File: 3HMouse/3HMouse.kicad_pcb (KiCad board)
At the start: 2 copper layers, 204.8 x 104.8 mm, 85 parts, among them J1 USB_C_Receptacle_USB2.0, SW1 CherryMX, SW10 CherryMX, SW11 CherryMX, SW12 CherryMX, SW13 CherryMX, SW14 CherryMX, SW15 CherryMX, SW16 CherryMX, SW17 CherryMX, SW18 CherryMX, SW19 CherryMX, SW2 CherryMX, SW20 CherryMX, SW21 CherryMX, SW22 CherryMX, SW23 CherryMX, SW24 CherryMX, SW25 CherryMX, SW26 CherryMX, SW27 CherryMX, SW28 CherryMX, SW29 CherryMX, SW3 CherryMX, SW30 RotaryEncoder, SW31 RotaryEncoder, SW4 CherryMX, SW5 CherryMX, SW6 CherryMX, SW7 CherryMX, SW8 CherryMX, SW9 CherryMX, U1 ATmega32U4-M, U2 USBLC6-2SC6, Y1 16 MHz

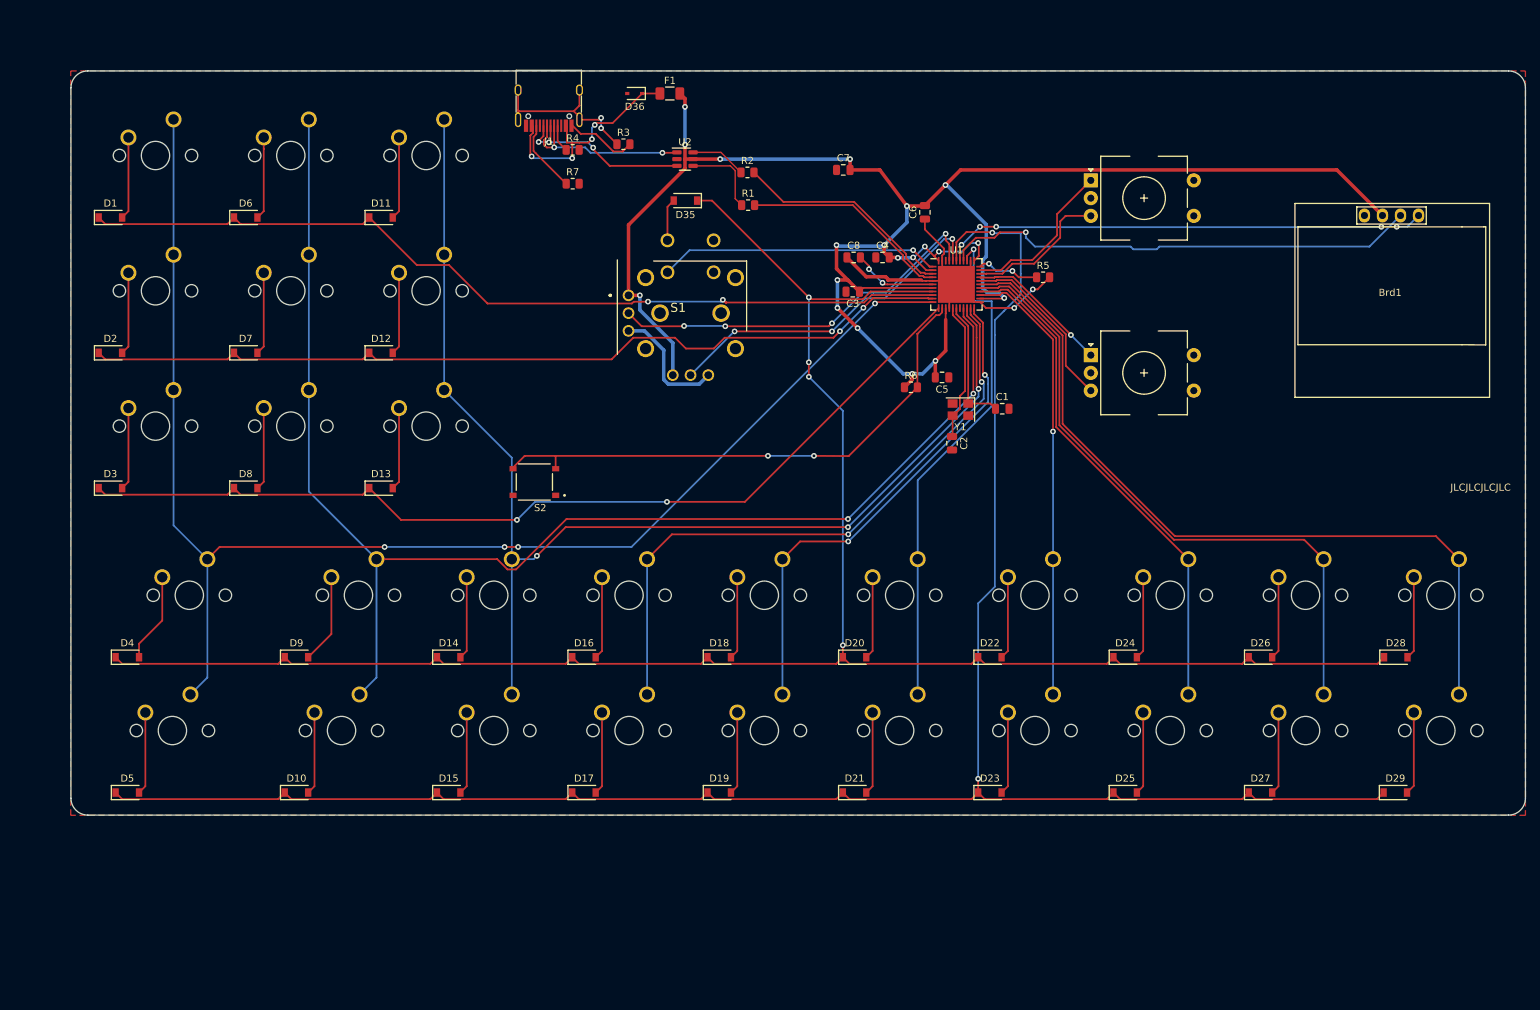
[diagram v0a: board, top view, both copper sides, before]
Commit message: Placements done for v2
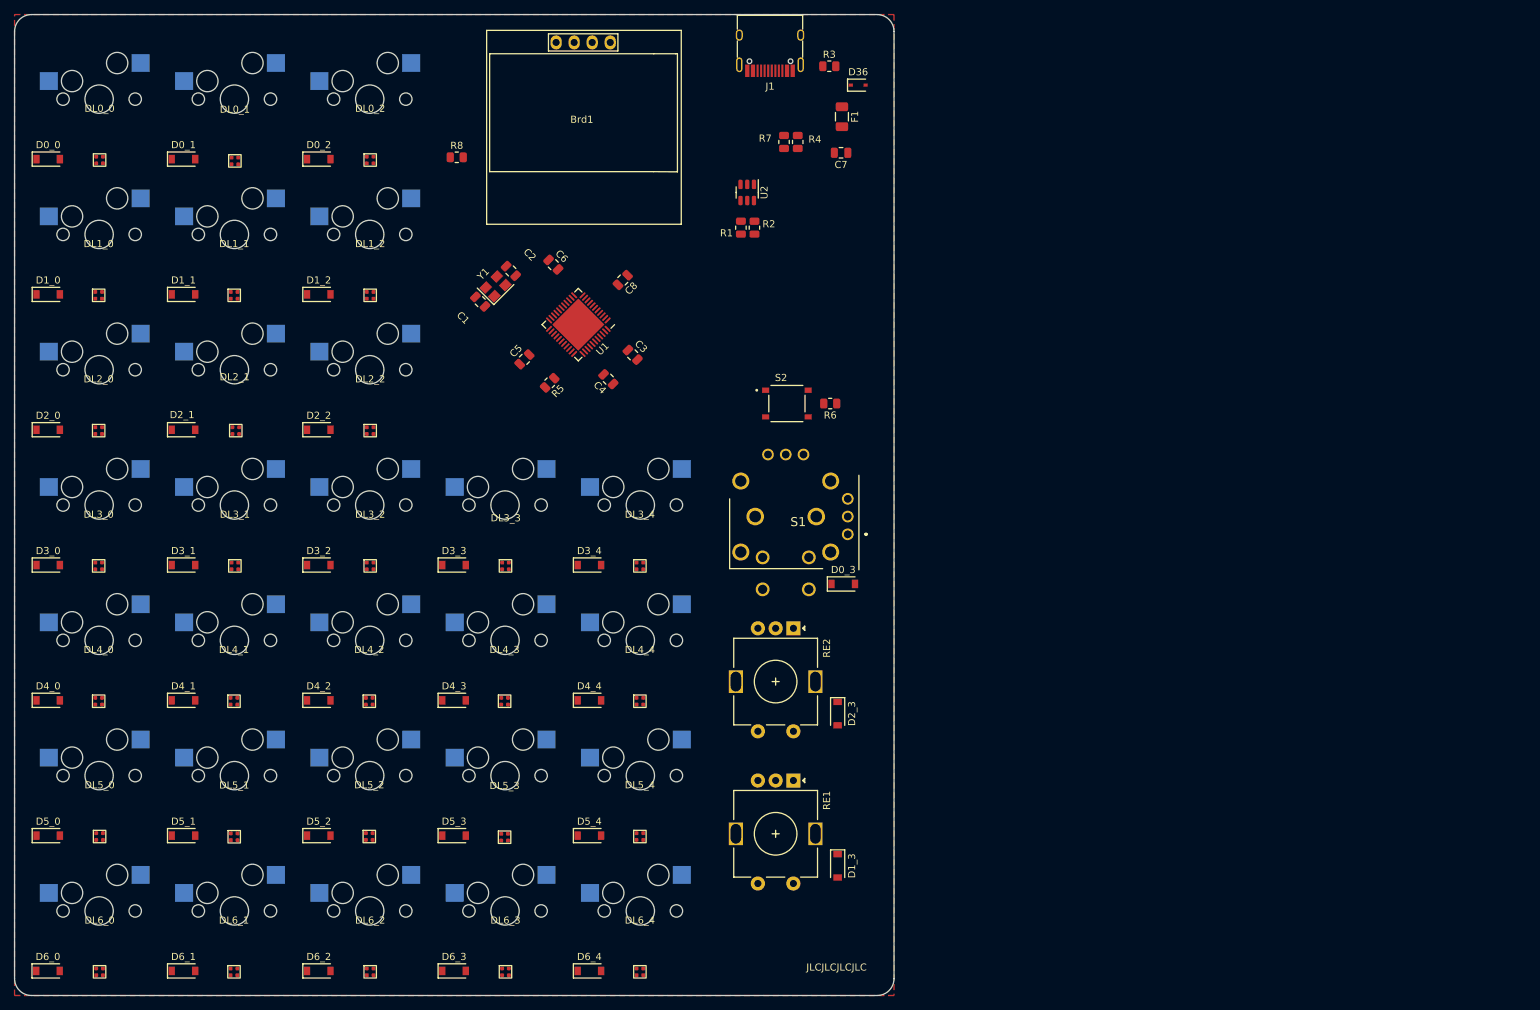
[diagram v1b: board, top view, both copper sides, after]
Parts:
- removed D1, D10, D11, D12, D13, D14, D15, D16, D17, D18, D19, D2, D20, D21, D22, D23, D24, D25, D26, D27, D28, D29, D3, D35, D4, D5, D6, D7, D8, D9: D_Small, Diode_SMD:D_SOD-123
- removed SW1, SW11, SW12, SW13, SW14, SW15, SW16, SW17, SW18, SW19, SW2, SW20, SW21, SW22, SW23, SW24, SW25, SW26, SW27, SW28, SW29, SW3, SW6, SW7, SW8, SW9: CherryMX, MX_Only:MXOnly-1U-NoLED
- removed SW10, SW5: CherryMX, MX_Only:MXOnly-1.25U-NoLED
- removed SW30, SW31: RotaryEncoder, Keebio-Parts:RotaryEncoder_EC11
- removed SW4: CherryMX, MX_Only:MXOnly-1.5U-NoLED
- added D0_0: D_Small, Diode_SMD:D_SOD-123, F.Cu at (26.2, 41.8)
- added D0_1: D_Small, Diode_SMD:D_SOD-123, F.Cu at (45.2, 41.8)
- added D0_2: D_Small, Diode_SMD:D_SOD-123, F.Cu at (64.3, 41.8)
- added D0_3: D_Small, Diode_SMD:D_SOD-123, F.Cu at (138.1, 101.6)
- added D1_0: D_Small, Diode_SMD:D_SOD-123, F.Cu at (26.2, 60.8)
- added D1_1: D_Small, Diode_SMD:D_SOD-123, F.Cu at (45.2, 60.8)
- added D1_2: D_Small, Diode_SMD:D_SOD-123, F.Cu at (64.3, 60.8)
- added D1_3: D_Small, Diode_SMD:D_SOD-123, F.Cu at (137.3, 141.3)
- added D2_0: D_Small, Diode_SMD:D_SOD-123, F.Cu at (26.2, 79.9)
- added D2_1: D_Small, Diode_SMD:D_SOD-123, F.Cu at (45.2, 79.9)
- added D2_2: D_Small, Diode_SMD:D_SOD-123, F.Cu at (64.3, 79.9)
- added D2_3: D_Small, Diode_SMD:D_SOD-123, F.Cu at (137.3, 119.9)
- added D3_0: D_Small, Diode_SMD:D_SOD-123, F.Cu at (26.2, 98.9)
- added D3_1: D_Small, Diode_SMD:D_SOD-123, F.Cu at (45.2, 98.9)
- added D3_2: D_Small, Diode_SMD:D_SOD-123, F.Cu at (64.3, 98.9)
- added D3_3: D_Small, Diode_SMD:D_SOD-123, F.Cu at (83.3, 98.9)
- added D3_4: D_Small, Diode_SMD:D_SOD-123, F.Cu at (102.4, 98.9)
- added D4_0: D_Small, Diode_SMD:D_SOD-123, F.Cu at (26.2, 118.0)
- added D4_1: D_Small, Diode_SMD:D_SOD-123, F.Cu at (45.2, 118.0)
- added D4_2: D_Small, Diode_SMD:D_SOD-123, F.Cu at (64.3, 118.0)
- added D4_3: D_Small, Diode_SMD:D_SOD-123, F.Cu at (83.3, 118.0)
- added D4_4: D_Small, Diode_SMD:D_SOD-123, F.Cu at (102.4, 118.0)
- added D5_0: D_Small, Diode_SMD:D_SOD-123, F.Cu at (26.2, 137.0)
- added D5_1: D_Small, Diode_SMD:D_SOD-123, F.Cu at (45.2, 137.0)
- added D5_2: D_Small, Diode_SMD:D_SOD-123, F.Cu at (64.3, 137.0)
- added D5_3: D_Small, Diode_SMD:D_SOD-123, F.Cu at (83.3, 137.0)
- added D5_4: D_Small, Diode_SMD:D_SOD-123, F.Cu at (102.4, 137.0)
- added D6_0: D_Small, Diode_SMD:D_SOD-123, F.Cu at (26.1, 156.1)
- added D6_1: D_Small, Diode_SMD:D_SOD-123, F.Cu at (45.2, 156.1)
- added D6_2: D_Small, Diode_SMD:D_SOD-123, F.Cu at (64.3, 156.1)
- added D6_3: D_Small, Diode_SMD:D_SOD-123, F.Cu at (83.3, 156.1)
- added D6_4: D_Small, Diode_SMD:D_SOD-123, F.Cu at (102.4, 156.1)
- added DL0_0: SK6805-EC15, HLibrary:SK6805-EC15, F.Cu at (33.4, 41.9)
- added DL0_1: SK6805-EC15, HLibrary:SK6805-EC15, F.Cu at (52.5, 42.0)
- added DL0_2: SK6805-EC15, HLibrary:SK6805-EC15, F.Cu at (71.5, 41.9)
- added DL1_0: SK6805-EC15, HLibrary:SK6805-EC15, F.Cu at (33.3, 61.0)
- added DL1_1: SK6805-EC15, HLibrary:SK6805-EC15, F.Cu at (52.4, 61.0)
- added DL1_2: SK6805-EC15, HLibrary:SK6805-EC15, F.Cu at (71.5, 61.0)
- added DL2_0: SK6805-EC15, HLibrary:SK6805-EC15, F.Cu at (33.3, 80.0)
- added DL2_1: SK6805-EC15, HLibrary:SK6805-EC15, F.Cu at (52.6, 80.0)
- added DL2_2: SK6805-EC15, HLibrary:SK6805-EC15, F.Cu at (71.5, 80.0)
- added DL3_0: SK6805-EC15, HLibrary:SK6805-EC15, F.Cu at (33.3, 99.1)
- added DL3_1: SK6805-EC15, HLibrary:SK6805-EC15, F.Cu at (52.5, 99.1)
- added DL3_2: SK6805-EC15, HLibrary:SK6805-EC15, F.Cu at (71.5, 99.1)
- added DL3_3: SK6805-EC15, HLibrary:SK6805-EC15, F.Cu at (90.6, 99.1)
- added DL3_4: SK6805-EC15, HLibrary:SK6805-EC15, F.Cu at (109.5, 99.1)
- added DL4_0: SK6805-EC15, HLibrary:SK6805-EC15, F.Cu at (33.3, 118.1)
- added DL4_1: SK6805-EC15, HLibrary:SK6805-EC15, F.Cu at (52.3, 118.1)
- added DL4_2: SK6805-EC15, HLibrary:SK6805-EC15, F.Cu at (71.4, 118.1)
- added DL4_3: SK6805-EC15, HLibrary:SK6805-EC15, F.Cu at (90.4, 118.1)
- added DL4_4: SK6805-EC15, HLibrary:SK6805-EC15, F.Cu at (109.5, 118.1)
- added DL5_0: SK6805-EC15, HLibrary:SK6805-EC15, F.Cu at (33.4, 137.2)
- added DL5_1: SK6805-EC15, HLibrary:SK6805-EC15, F.Cu at (52.4, 137.2)
- added DL5_2: SK6805-EC15, HLibrary:SK6805-EC15, F.Cu at (71.4, 137.2)
- added DL5_3: SK6805-EC15, HLibrary:SK6805-EC15, F.Cu at (90.4, 137.3)
- added DL5_4: SK6805-EC15, HLibrary:SK6805-EC15, F.Cu at (109.5, 137.2)
- added DL6_0: SK6805-EC15, HLibrary:SK6805-EC15, F.Cu at (33.4, 156.2)
- added DL6_1: SK6805-EC15, HLibrary:SK6805-EC15, F.Cu at (52.3, 156.2)
- added DL6_2: SK6805-EC15, HLibrary:SK6805-EC15, F.Cu at (71.5, 156.2)
- added DL6_3: SK6805-EC15, HLibrary:SK6805-EC15, F.Cu at (90.6, 156.2)
- added DL6_4: SK6805-EC15, HLibrary:SK6805-EC15, F.Cu at (109.5, 156.2)
- added R8: 500, Resistor_SMD:R_0805_2012Metric, F.Cu at (83.7, 41.5)
- added RE1: RotaryEncoder_Switch, Rotary_Encoder:RotaryEncoder_Alps_EC11E-Switch_Vertical_H20mm, F.Cu at (131.1, 129.3)
- added RE2: RotaryEncoder_Switch, Rotary_Encoder:RotaryEncoder_Alps_EC11E-Switch_Vertical_H20mm, F.Cu at (131.1, 107.8)
- added SW0_0: CherryMX, MX_Only:MXOnly-1U-Hotswap, F.Cu at (33.3, 33.3)
- added SW0_1: CherryMX, MX_Only:MXOnly-1U-Hotswap, F.Cu at (52.4, 33.3)
- added SW0_2: CherryMX, MX_Only:MXOnly-1U-Hotswap, F.Cu at (71.4, 33.3)
- added SW1_0: CherryMX, MX_Only:MXOnly-1U-Hotswap, F.Cu at (33.3, 52.4)
- added SW1_1: CherryMX, MX_Only:MXOnly-1U-Hotswap, F.Cu at (52.4, 52.4)
- added SW1_2: CherryMX, MX_Only:MXOnly-1U-Hotswap, F.Cu at (71.4, 52.4)
- added SW2_0: CherryMX, MX_Only:MXOnly-1U-Hotswap, F.Cu at (33.3, 71.4)
- added SW2_1: CherryMX, MX_Only:MXOnly-1U-Hotswap, F.Cu at (52.4, 71.4)
- added SW2_2: CherryMX, MX_Only:MXOnly-1U-Hotswap, F.Cu at (71.4, 71.4)
- added SW3_0: CherryMX, MX_Only:MXOnly-1U-Hotswap, F.Cu at (33.3, 90.5)
- added SW3_1: CherryMX, MX_Only:MXOnly-1U-Hotswap, F.Cu at (52.4, 90.5)
- added SW3_2: CherryMX, MX_Only:MXOnly-1U-Hotswap, F.Cu at (71.4, 90.5)
- added SW3_3: CherryMX, MX_Only:MXOnly-1U-Hotswap, F.Cu at (90.5, 90.5)
- added SW3_4: CherryMX, MX_Only:MXOnly-1U-Hotswap, F.Cu at (109.5, 90.5)
- added SW4_0: CherryMX, MX_Only:MXOnly-1U-Hotswap, F.Cu at (33.3, 109.5)
- added SW4_1: CherryMX, MX_Only:MXOnly-1U-Hotswap, F.Cu at (52.4, 109.5)
- added SW4_2: CherryMX, MX_Only:MXOnly-1U-Hotswap, F.Cu at (71.4, 109.5)
- added SW4_3: CherryMX, MX_Only:MXOnly-1U-Hotswap, F.Cu at (90.5, 109.5)
- added SW4_4: CherryMX, MX_Only:MXOnly-1U-Hotswap, F.Cu at (109.5, 109.5)
- added SW5_0: CherryMX, MX_Only:MXOnly-1U-Hotswap, F.Cu at (33.3, 128.6)
- added SW5_1: CherryMX, MX_Only:MXOnly-1U-Hotswap, F.Cu at (52.4, 128.6)
- added SW5_2: CherryMX, MX_Only:MXOnly-1U-Hotswap, F.Cu at (71.4, 128.6)
- added SW5_3: CherryMX, MX_Only:MXOnly-1U-Hotswap, F.Cu at (90.5, 128.6)
- added SW5_4: CherryMX, MX_Only:MXOnly-1U-Hotswap, F.Cu at (109.5, 128.6)
- added SW6_0: CherryMX, MX_Only:MXOnly-1U-Hotswap, F.Cu at (33.3, 147.6)
- added SW6_1: CherryMX, MX_Only:MXOnly-1U-Hotswap, F.Cu at (52.4, 147.6)
- added SW6_2: CherryMX, MX_Only:MXOnly-1U-Hotswap, F.Cu at (71.4, 147.6)
- added SW6_3: CherryMX, MX_Only:MXOnly-1U-Hotswap, F.Cu at (90.5, 147.6)
- added SW6_4: CherryMX, MX_Only:MXOnly-1U-Hotswap, F.Cu at (109.5, 147.6)
- moved Brd1 116.4 mm to (101.3, 36.0)
- moved C1 75.0 mm to (87.0, 61.8), turned to 135 degrees
- moved R5 71.0 mm to (96.8, 73.3), turned to -135 degrees
- moved Y1 67.7 mm to (89.2, 59.7), turned to 45 degrees
- moved C2 66.7 mm to (91.3, 57.5), turned to -45 degrees
- moved C5 58.9 mm to (93.2, 70.0), turned to 45 degrees
- moved U1 53.5 mm to (100.8, 65.1), turned to -135 degrees
- moved C6 52.8 mm to (97.3, 56.6), turned to -45 degrees
- moved S1 45.7 mm to (138.7, 94.6), turned to 0 degrees
- moved C4 42.2 mm to (105.0, 72.8), turned to 135 degrees
- moved S2 37.2 mm to (130.2, 76.2), turned to 0 degrees
- moved C8 32.7 mm to (107.1, 58.8), turned to -135 degrees
- moved C3 32.2 mm to (108.5, 69.3), turned to -45 degrees
- moved J1 32.1 mm to (127.8, 26.2)
- moved R4 31.7 mm to (131.7, 39.4), turned to -90 degrees
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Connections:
- S1 pad C1: COL10 -> COL3
- U1 pad 1: COL10 -> unconnected-(U1-Pad1)
- U1 pad 18: unconnected-(U1-Pad18) -> LED
- U1 pad 25: COL6 -> ROW6
- U1 pad 26: COL7 -> unconnected-(U1-Pad26)
- U1 pad 27: COL8 -> unconnected-(U1-Pad27)
- U1 pad 28: COL9 -> ROW5
- U1 pad 36: COL5 -> unconnected-(U1-Pad36)
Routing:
- net ROW4: track 279.0 -> 0.00 mm, vias 2 -> 0
- net ROW3: track 277.5 -> 0.00 mm, vias 4 -> 0
- net +5V: track 270.7 -> 0.00 mm, vias 20 -> 0
- net COL0: track 201.0 -> 0.00 mm, vias 4 -> 0
- net COL1: track 193.4 -> 0.00 mm, vias 2 -> 0
- net COL2: track 173.2 -> 0.00 mm, vias 3 -> 0
- net ROW2: track 134.0 -> 0.00 mm, vias 2 -> 0
- net ROW0: track 124.9 -> 0.00 mm, vias 2 -> 0
- net ROW1: track 124.2 -> 0.00 mm, vias 2 -> 0
- net COL9: track 109.9 -> 0.00 mm
- net COL8: track 90.7 -> 0.00 mm
- net COL3: track 89.3 -> 0.00 mm, vias 2 -> 0
- net GND: track 79.9 -> 0.00 mm, vias 2 -> 0
- net /RESET: track 76.7 -> 0.00 mm, vias 2 -> 0
- net COL7: track 71.5 -> 0.00 mm
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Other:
- board size 204.8 x 104.8 mm -> 123.8 x 138.1 mm
